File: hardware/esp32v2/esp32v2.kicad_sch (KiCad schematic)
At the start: 10 parts, among them J1 Conn_01x01, J2 Conn_01x02, J3 Conn_01x10, J6 Conn_01x01, U2 ESP32-S3-MINI-1-N8

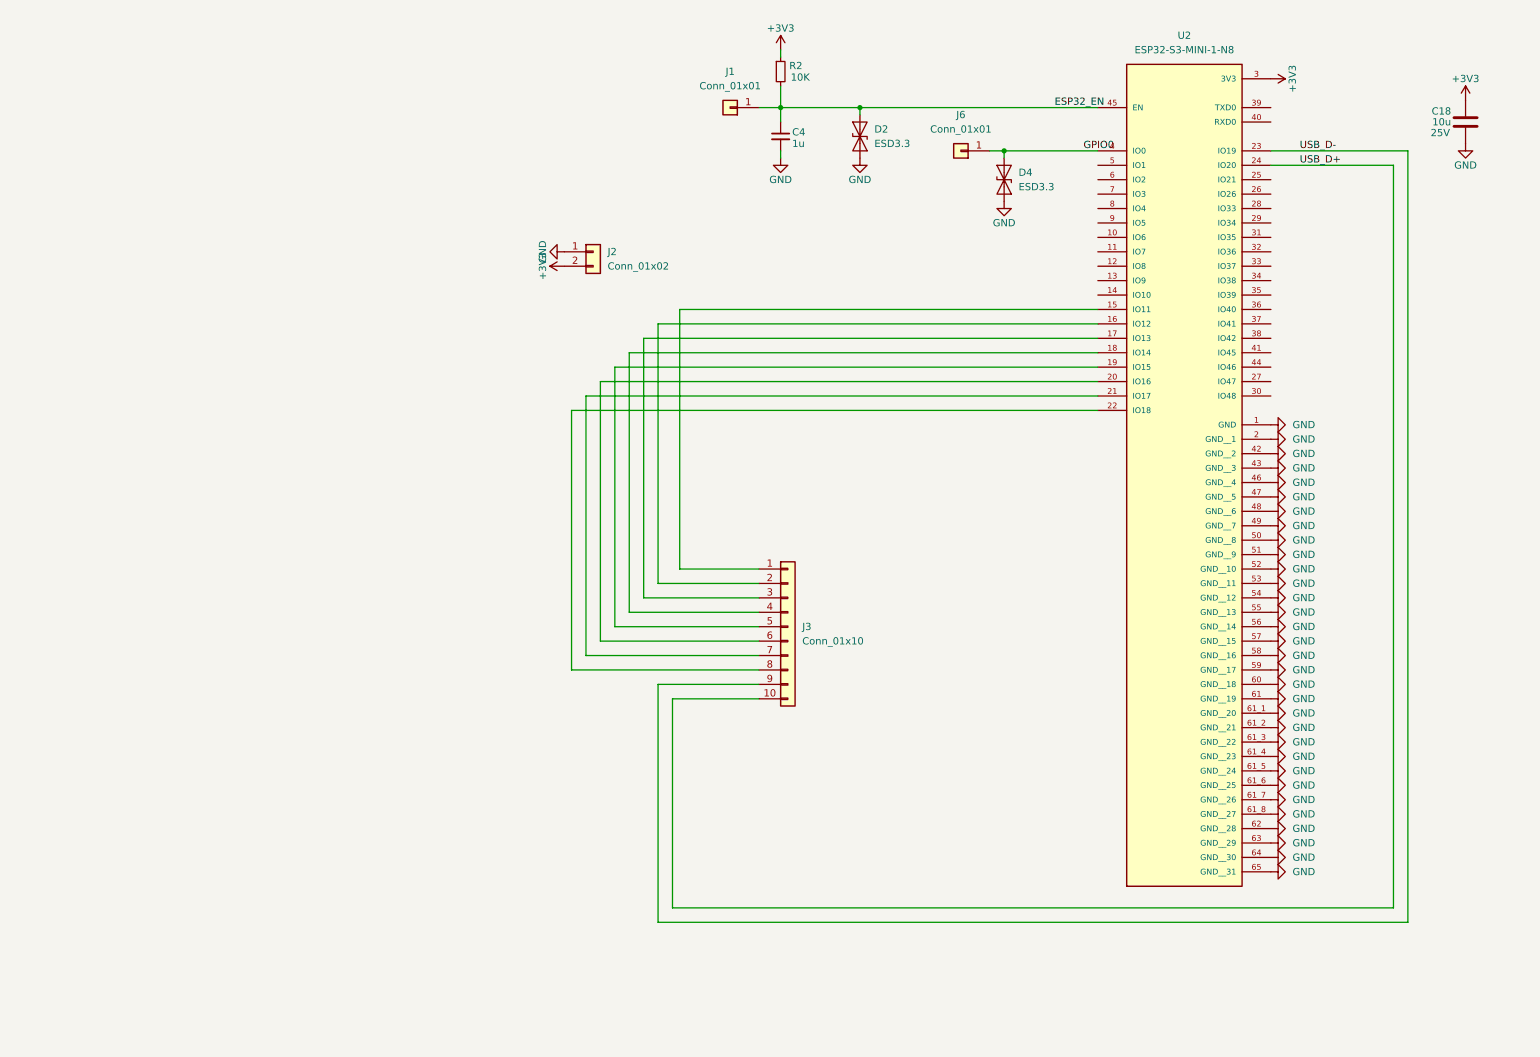
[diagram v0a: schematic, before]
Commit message: wip
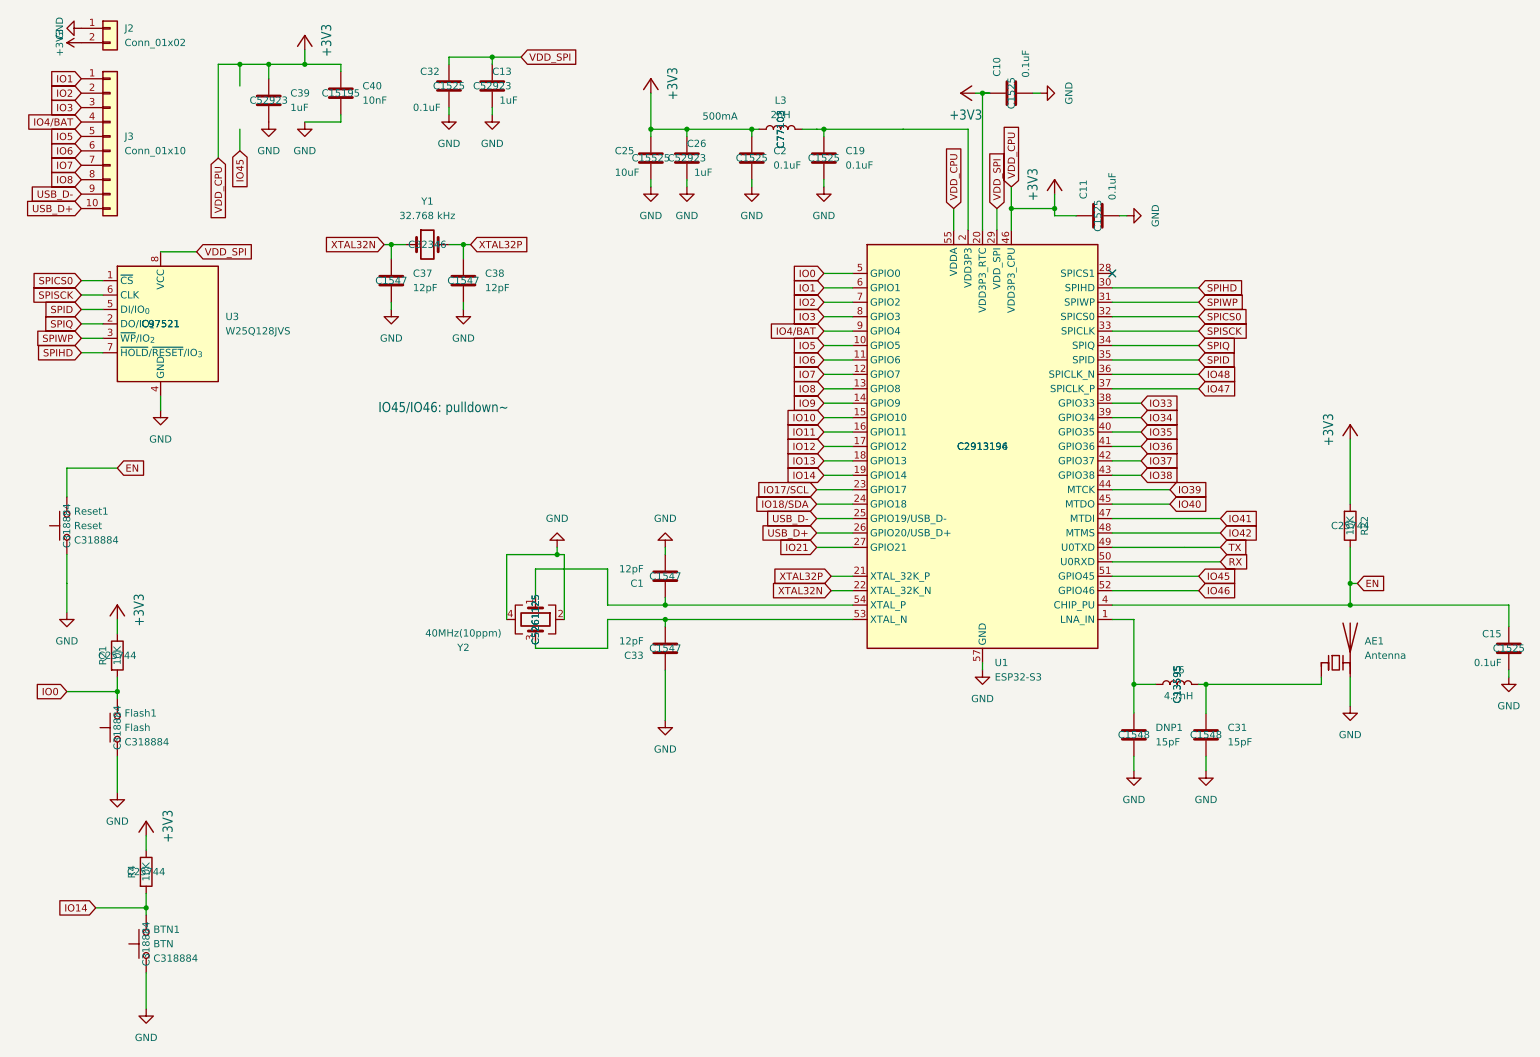
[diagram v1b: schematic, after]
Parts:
- removed C18: 10u, Capacitor_SMD:C_0603_1608Metric, symbol Device:C
- removed C4: 1u, Capacitor_SMD:C_0603_1608Metric, symbol Morten_Library.kicad_sym_9:C_Small
- removed D2, D4: ESD3.3, Package_TO_SOT_SMD:SOT-723, symbol Morten_Library.kicad_sym_9:ESD9B3.3ST5G
- removed J1, J6: Conn_01x01, Connector_PinHeader_1.00mm:PinHeader_1x01_P1.00mm_Vertical, symbol Connector_Generic:Conn_01x01
- removed R2: 10K, Resistor_SMD:R_0402_1005Metric, symbol Morten_Library.kicad_sym_9:R_Small
- removed U2: ESP32-S3-MINI-1-N8, ESP32_S3_MINI_1_N8:XCVR_ESP32-S3-MINI-1-N8, symbol ESP32-S3-MINI-1-N8:ESP32-S3-MINI-1-N8
- added AE1: Antenna, RF_Antenna:Texas_SWRA117D_2.4GHz_Left, symbol Device:Antenna_Chip
- added BTN1: BTN, Button_Switch_SMD:SW_Push_1P1T_XKB_TS-1187A, symbol Switch:SW_Push
- added C1, C33, C37, C38: 12pF, Capacitor_SMD:C_0201_0603Metric, symbol Device:C
- added C10, C11, C15, C19, C2, C32: 0.1uF, Capacitor_SMD:C_0201_0603Metric, symbol Device:C
- added C13, C26, C39: 1uF, Capacitor_SMD:C_0201_0603Metric, symbol Device:C
- added C25: 10uF, Capacitor_SMD:C_0201_0603Metric, symbol Device:C
- added C31, DNP1: 15pF, Capacitor_SMD:C_0201_0603Metric, symbol Device:C
- added C40: 10nF, Capacitor_SMD:C_0201_0603Metric, symbol Device:C
- added Flash1: Flash, Button_Switch_SMD:SW_Push_1P1T_XKB_TS-1187A, symbol Switch:SW_Push
- added L3: 2nH, Inductor_SMD:L_0201_0603Metric, symbol Device:L
- added L6: 4.7nH, Inductor_SMD:L_0201_0603Metric, symbol Device:L
- added R21, R22, R4: 10K, Resistor_SMD:R_0201_0603Metric, symbol Device:R
- added Reset1: Reset, Button_Switch_SMD:SW_Push_1P1T_XKB_TS-1187A, symbol Switch:SW_Push
- added U1: ESP32-S3, Package_DFN_QFN:QFN-56-1EP_7x7mm_P0.4mm_EP4x4mm, symbol MCU_Espressif:ESP32-S3
- added U3: W25Q128JVS, Package_SO:SOIC-8_5.3x5.3mm_P1.27mm, symbol Memory_Flash:W25Q128JVS
- added Y1: 32.768 kHz, Crystal:Crystal_SMD_3215-2Pin_3.2x1.5mm, symbol Device:Crystal
- added Y2: 40MHz(10ppm), Crystal:Crystal_SMD_2520-4Pin_2.5x2.0mm, symbol Device:Crystal_GND24
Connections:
- net +3V3: now also C10.1, C11.1, C2.1, C25.1, C26.1, C39.1, C40.1, L3.1, R21.1, R22.2, R4.1, U1.20 (VDD3P3_RTC), U1.46 (VDD3P3_CPU), U1.55 (VDDA), U1.56 (VDDA)
- net GND: now also AE1.2 (PCB_Trace), BTN1.1, C1.2, C10.2, C11.2, C13.2, C15.2, C19.2, C2.2, C25.2, C26.2, C31.2, C32.2, C33.1, C37.2, C38.2, C39.2, C40.2, DNP1.2, Flash1.1, Reset1.1, U1.57 (GND), U3.4 (GND), Y2.2, Y2.4
- net USB_D+: now also U1.26 (GPIO20/USB_D+)
- net USB_D-: now also U1.25 (GPIO19/USB_D-)
- net IO1: now reaches J3.1 (Pin_1)
- net IO1: now also U1.6 (GPIO1)
- net IO2: now reaches J3.2 (Pin_2)
- net IO2: now also U1.7 (GPIO2)
- net IO3: now reaches J3.3 (Pin_3)
- net IO3: now also U1.8 (GPIO3)
- net IO4/BAT: now reaches J3.4 (Pin_4)
- net IO4/BAT: now also U1.9 (GPIO4)
- net IO5: now reaches J3.5 (Pin_5)
- net IO5: now also U1.10 (GPIO5)
- net IO6: now reaches J3.6 (Pin_6)
- net IO6: now also U1.11 (GPIO6)
- net IO7: now reaches J3.7 (Pin_7)
- net IO7: now also U1.12 (GPIO7)
- net IO8: now reaches J3.8 (Pin_8)
- net IO8: now also U1.13 (GPIO8)
- new net: AE1.1 (FEED), C31.1, L6.2
- new net: DNP1.1, L6.1, U1.1 (LNA_IN)
- new net: C1.1, U1.54 (XTAL_P), Y2.1
- new net: C19.1, L3.2, U1.2 (VDD3P3), U1.3 (VDD3P3)
- new net: C33.2, U1.53 (XTAL_N), Y2.3
- new net EN: C15.1, R22.1, Reset1.2, U1.4 (CHIP_PU)
- new net IO0: Flash1.2, R21.2, U1.5 (GPIO0)
- new net IO10: U1.15 (GPIO10)
- new net IO11: U1.16 (GPIO11)
- new net IO12: U1.17 (GPIO12)
- new net IO13: U1.18 (GPIO13)
- new net IO14: BTN1.2, R4.2, U1.19 (GPIO14)
- new net IO17/SCL: U1.23 (GPIO17)
- new net IO18/SDA: U1.24 (GPIO18)
- new net IO21: U1.27 (GPIO21)
- new net IO33: U1.38 (GPIO33)
- new net IO34: U1.39 (GPIO34)
- new net IO35: U1.40 (GPIO35)
- new net IO36: U1.41 (GPIO36)
- new net IO37: U1.42 (GPIO37)
- new net IO38: U1.43 (GPIO38)
- new net IO39: U1.44 (MTCK)
- new net IO40: U1.45 (MTDO)
- new net IO41: U1.47 (MTDI)
- new net IO42: U1.48 (MTMS)
- new net IO45: U1.51 (GPIO45)
- new net IO46: U1.52 (GPIO46)
- new net IO47: U1.37 (SPICLK_P)
- new net IO48: U1.36 (SPICLK_N)
- new net IO9: U1.14 (GPIO9)
- new net RX: U1.50 (U0RXD)
- new net SPICS0: U1.32 (SPICS0), U3.1 (~{CS})
- new net SPID: U1.35 (SPID), U3.5 (DI/IO_{0})
- new net SPIHD: U1.30 (SPIHD), U3.7 (~{HOLD}/~{RESET}/IO_{3})
- new net SPIQ: U1.34 (SPIQ), U3.2 (DO/IO_{1})
- new net SPISCK: U1.33 (SPICLK), U3.6 (CLK)
- new net SPIWP: U1.31 (SPIWP), U3.3 (~{WP}/IO_{2})
- new net TX: U1.49 (U0TXD)
- new net VDD_SPI: C13.1, C32.1, U1.29 (VDD_SPI), U3.8 (VCC)
- new net XTAL32N: C37.1, U1.22 (XTAL_32K_N), Y1.1
- new net XTAL32P: C38.1, U1.21 (XTAL_32K_P), Y1.2
- no-connect marks 0 -> 1
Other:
- note added: "500mA"
- note added: "IO45/IO46: pulldown~~{}"
- moved on the sheet: J2, J3

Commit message: wip
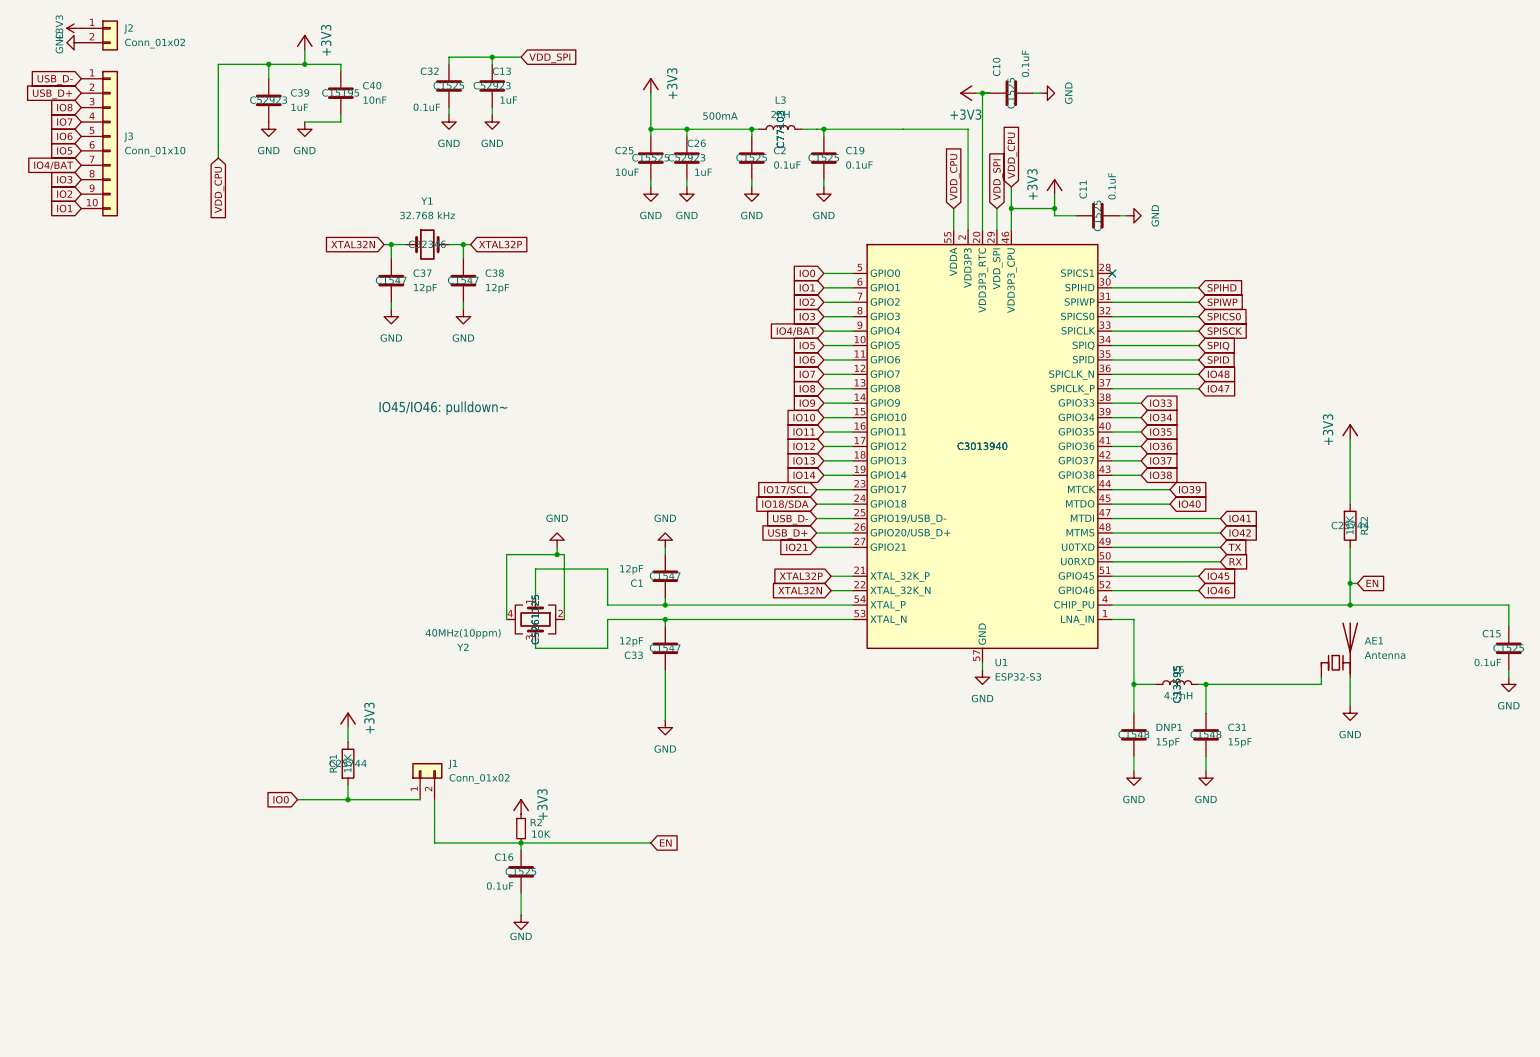
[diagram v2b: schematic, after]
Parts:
- removed BTN1: BTN, Button_Switch_SMD:SW_Push_1P1T_XKB_TS-1187A, symbol Switch:SW_Push
- removed Flash1: Flash, Button_Switch_SMD:SW_Push_1P1T_XKB_TS-1187A, symbol Switch:SW_Push
- removed R4: 10K, Resistor_SMD:R_0201_0603Metric, symbol Device:R
- removed Reset1: Reset, Button_Switch_SMD:SW_Push_1P1T_XKB_TS-1187A, symbol Switch:SW_Push
- removed U3: W25Q128JVS, Package_SO:SOIC-8_5.3x5.3mm_P1.27mm, symbol Memory_Flash:W25Q128JVS
- added C16: 0.1uF, Capacitor_SMD:C_0201_0603Metric, symbol Device:C
- added J1: Conn_01x02, Connector_JST:JST_SH_BM02B-SRSS-TB_1x02-1MP_P1.00mm_Vertical, symbol Connector_Generic:Conn_01x02
- added R2: 10K, Resistor_SMD:R_0201_0603Metric, symbol Morten_Library.kicad_sym_9:R_Small
- U1: LCSC C2913194 -> C3013940; MNF PART NUMBER C2913196 -> C3013940
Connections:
- net +3V3: now also J2.1 (Pin_1), R2.1; no longer J2.2 (Pin_2)
- net EN: now also C16.1, J1.2 (Pin_2), R2.2
- net GND: now also J2.2 (Pin_2), C16.2; no longer J2.1 (Pin_1)
- net IO0: now also J1.1 (Pin_1)
- net IO1: now also J3.10 (Pin_10); no longer J3.1 (Pin_1)
- net IO2: now also J3.9 (Pin_9); no longer J3.2 (Pin_2)
- net IO3: now also J3.8 (Pin_8); no longer J3.3 (Pin_3)
- net IO4/BAT: now also J3.7 (Pin_7); no longer J3.4 (Pin_4)
- net IO5: now also J3.6 (Pin_6); no longer J3.5 (Pin_5)
- net IO6: now also J3.5 (Pin_5); no longer J3.6 (Pin_6)
- net IO7: now also J3.4 (Pin_4); no longer J3.7 (Pin_7)
- net IO8: now also J3.3 (Pin_3); no longer J3.8 (Pin_8)
- net USB_D+: now also J3.2 (Pin_2); no longer J3.10 (Pin_10)
- net USB_D-: now also J3.1 (Pin_1); no longer J3.9 (Pin_9)
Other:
- moved on the sheet: R21

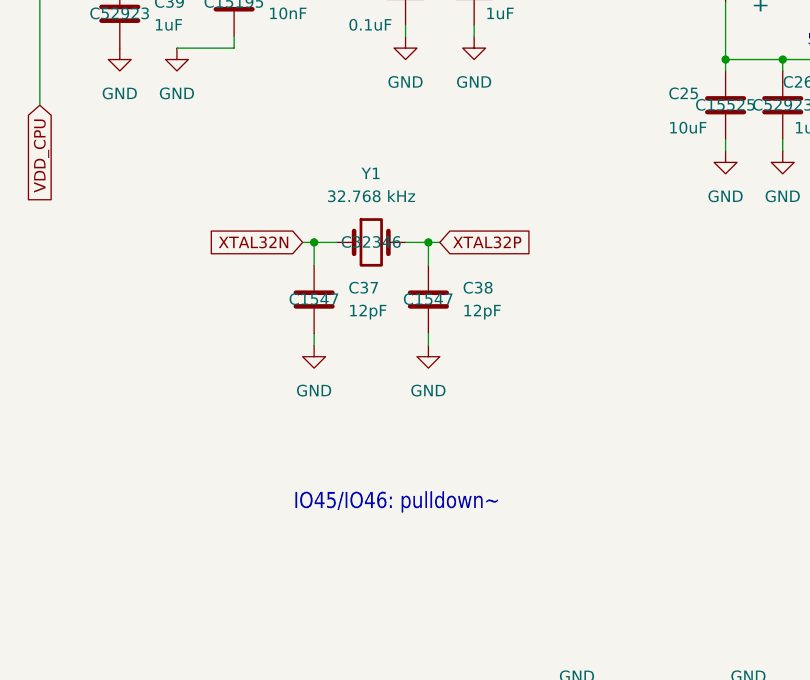
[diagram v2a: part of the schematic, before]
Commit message: wip
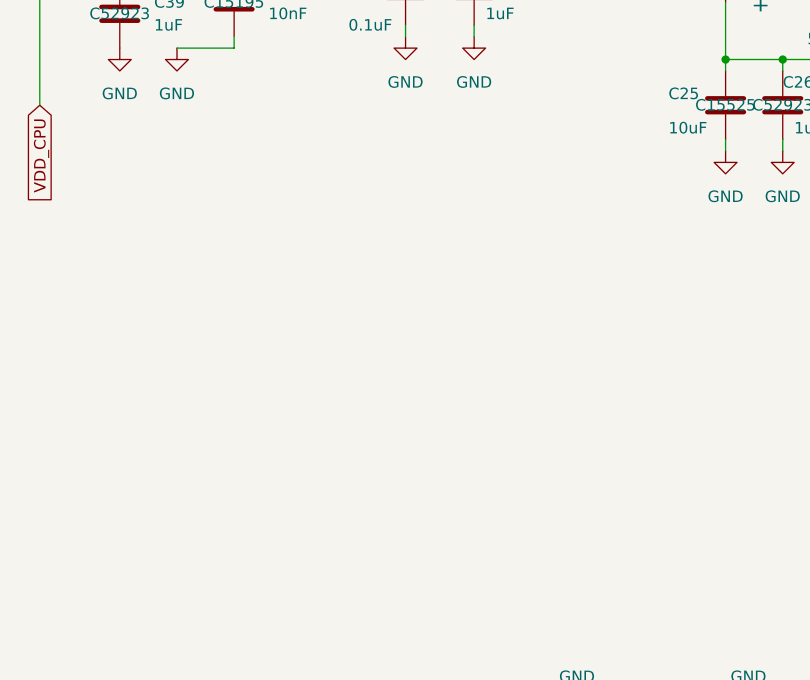
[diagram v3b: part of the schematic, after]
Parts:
- removed C37, C38: 12pF, Capacitor_SMD:C_0201_0603Metric, symbol Device:C
- removed Y1: 32.768 kHz, Crystal:Crystal_SMD_3215-2Pin_3.2x1.5mm, symbol Device:Crystal
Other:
- note removed: "IO45/IO46: pulldown~~{}"

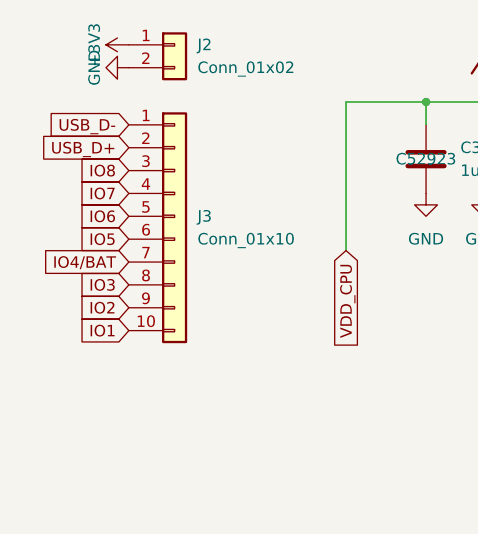
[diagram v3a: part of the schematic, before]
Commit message: wip esp32 v2
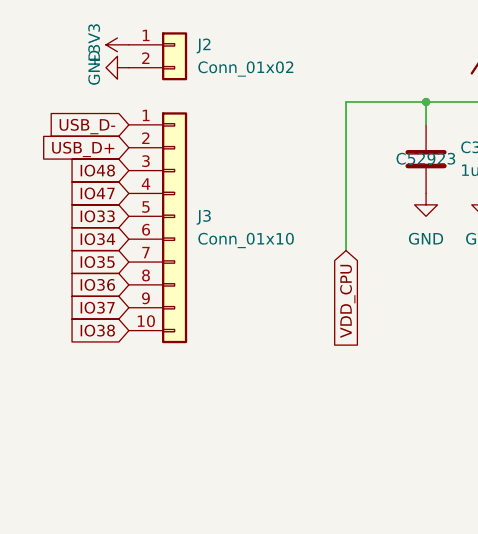
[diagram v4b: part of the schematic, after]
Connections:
- net IO1: no longer J3.10 (Pin_10)
- net IO2: no longer J3.9 (Pin_9)
- net IO3: no longer J3.8 (Pin_8)
- net IO33: now also J3.5 (Pin_5)
- net IO34: now also J3.6 (Pin_6)
- net IO35: now also J3.7 (Pin_7)
- net IO36: now also J3.8 (Pin_8)
- net IO37: now also J3.9 (Pin_9)
- net IO38: now also J3.10 (Pin_10)
- net IO47: now also J3.4 (Pin_4)
- net IO48: now also J3.3 (Pin_3)
- net IO4/BAT: no longer J3.7 (Pin_7)
- net IO5: no longer J3.6 (Pin_6)
- net IO6: no longer J3.5 (Pin_5)
- net IO7: no longer J3.4 (Pin_4)
- net IO8: no longer J3.3 (Pin_3)
